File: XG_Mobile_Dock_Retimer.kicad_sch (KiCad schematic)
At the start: 273 parts, among them J1 5-1775443-8, J13 39301240, J14 469911008, J2 20455-040E-76, J3 20455-040E-76, J7 CEE016400140111, SW1 SW_Push, U1 DS160PT801ACBR, U2 TPS7A8400ARGRR, U7 TPS7A8400ARGRR

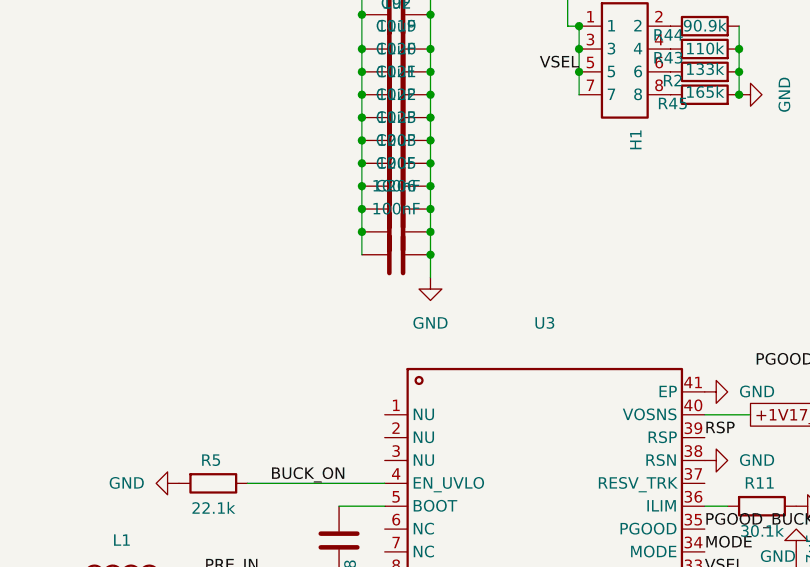
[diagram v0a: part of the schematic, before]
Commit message: ee
eee
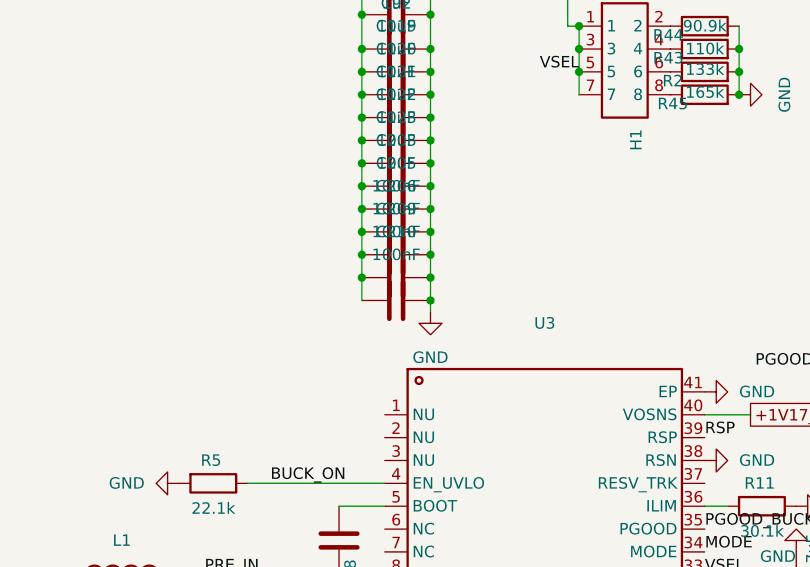
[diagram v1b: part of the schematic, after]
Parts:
- added C209, C210: 100nF, Capacitor_SMD:C_0201_0603Metric, symbol Device:C
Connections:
- net +1V17_2: now also C209.2, C210.2
- net GND: now also C209.1, C210.1

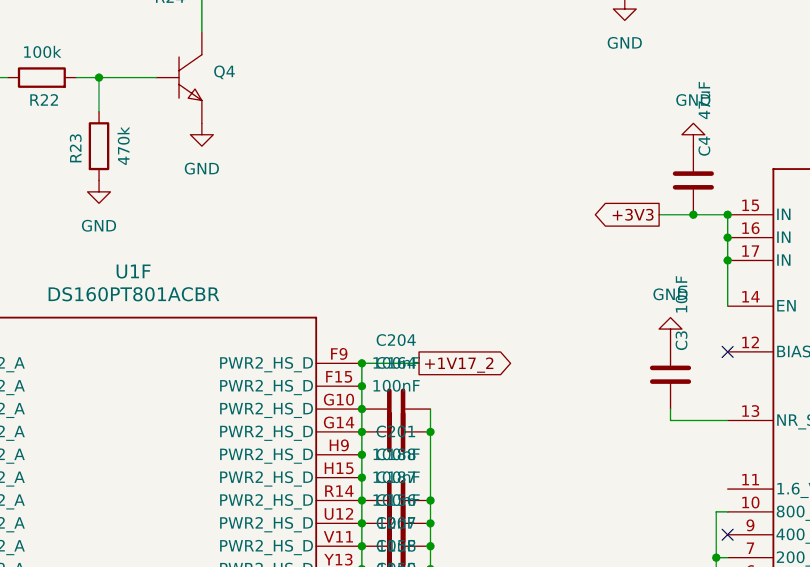
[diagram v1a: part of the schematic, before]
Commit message: eeee
eee
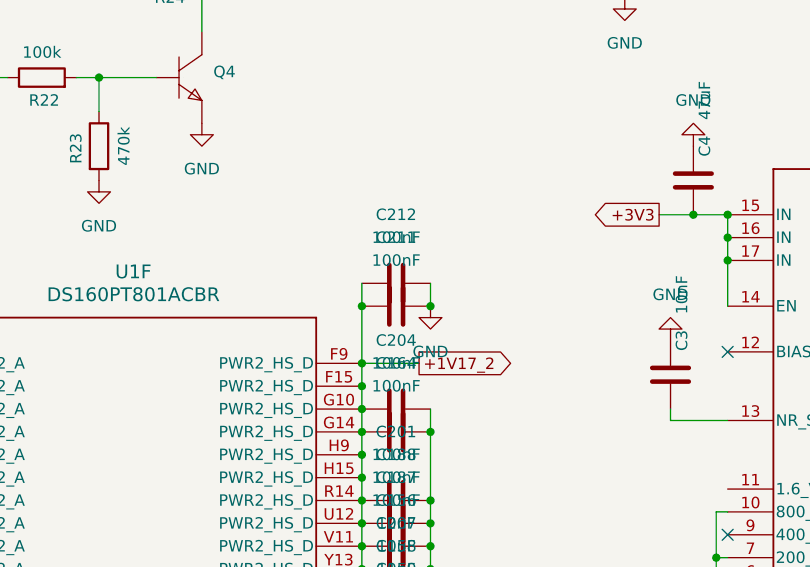
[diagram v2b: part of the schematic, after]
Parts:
- added C211, C212: 100nF, Capacitor_SMD:C_0201_0603Metric, symbol Device:C
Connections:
- net +1V17_2: now also C211.2, C212.2
- net GND: now also C211.1, C212.1

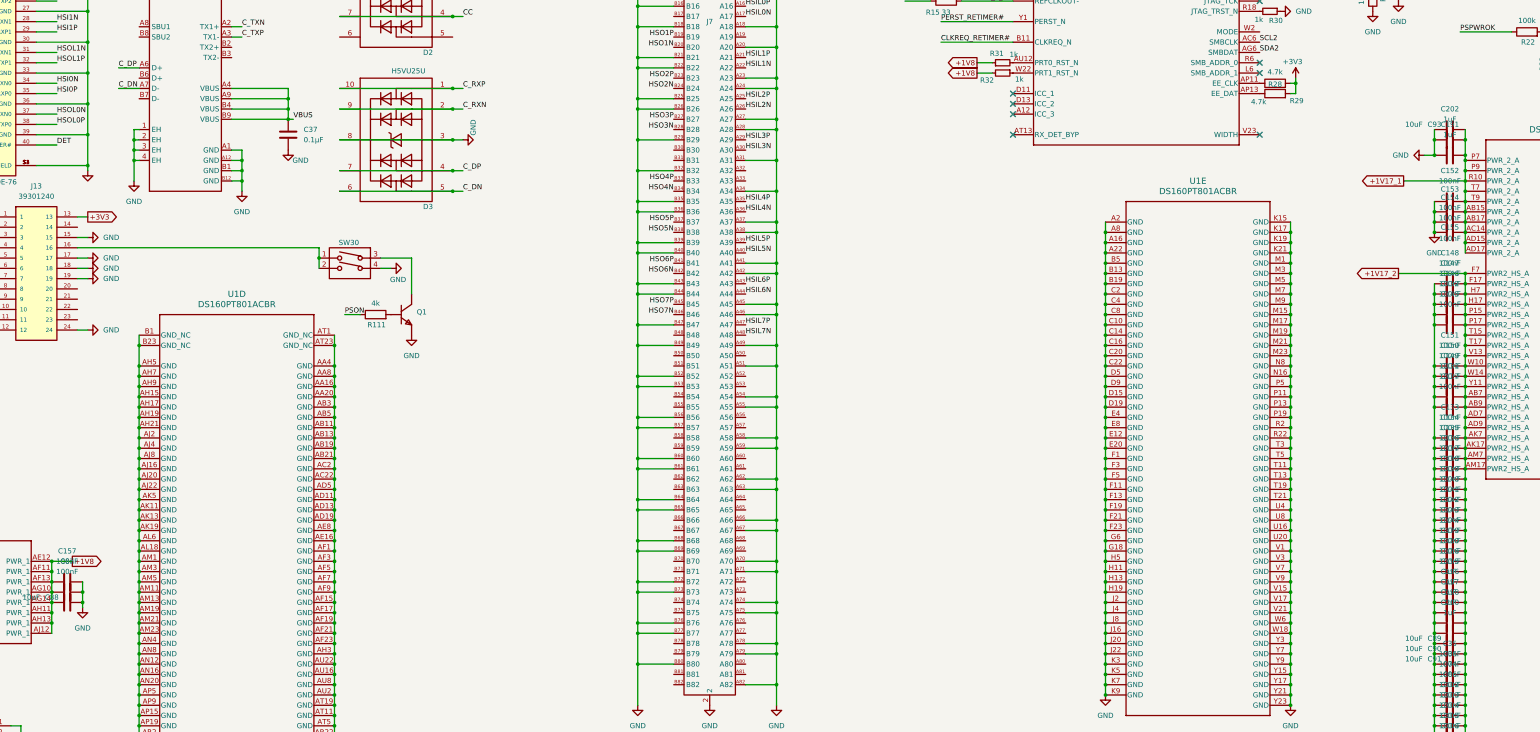
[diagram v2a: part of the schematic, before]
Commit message: eeeeee
eeeeee
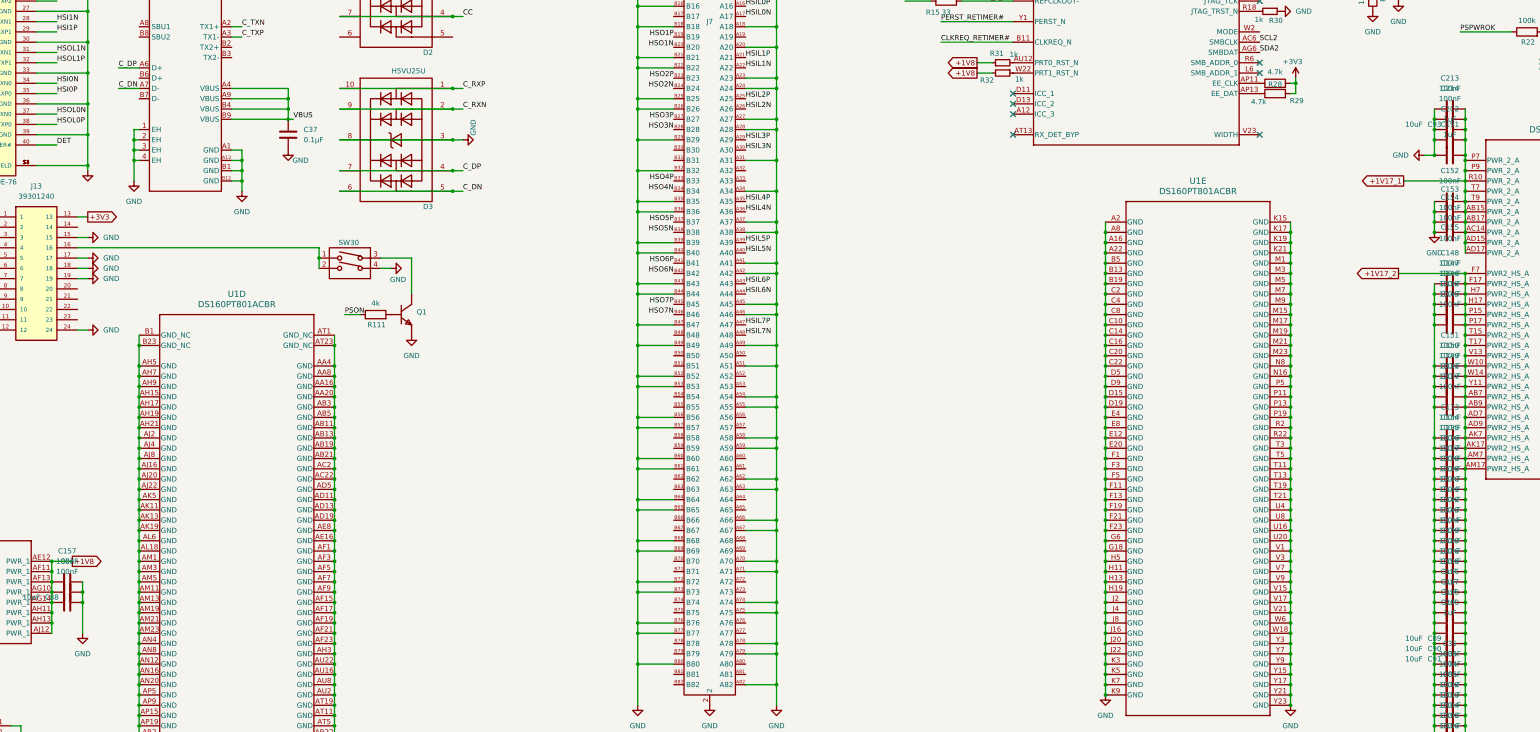
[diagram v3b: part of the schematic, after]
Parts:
- added C213, C214: 100nF, Capacitor_SMD:C_0201_0603Metric, symbol Device:C
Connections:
- net +1V17_1: now also C213.1, C214.1
- net GND: now also C213.2, C214.2

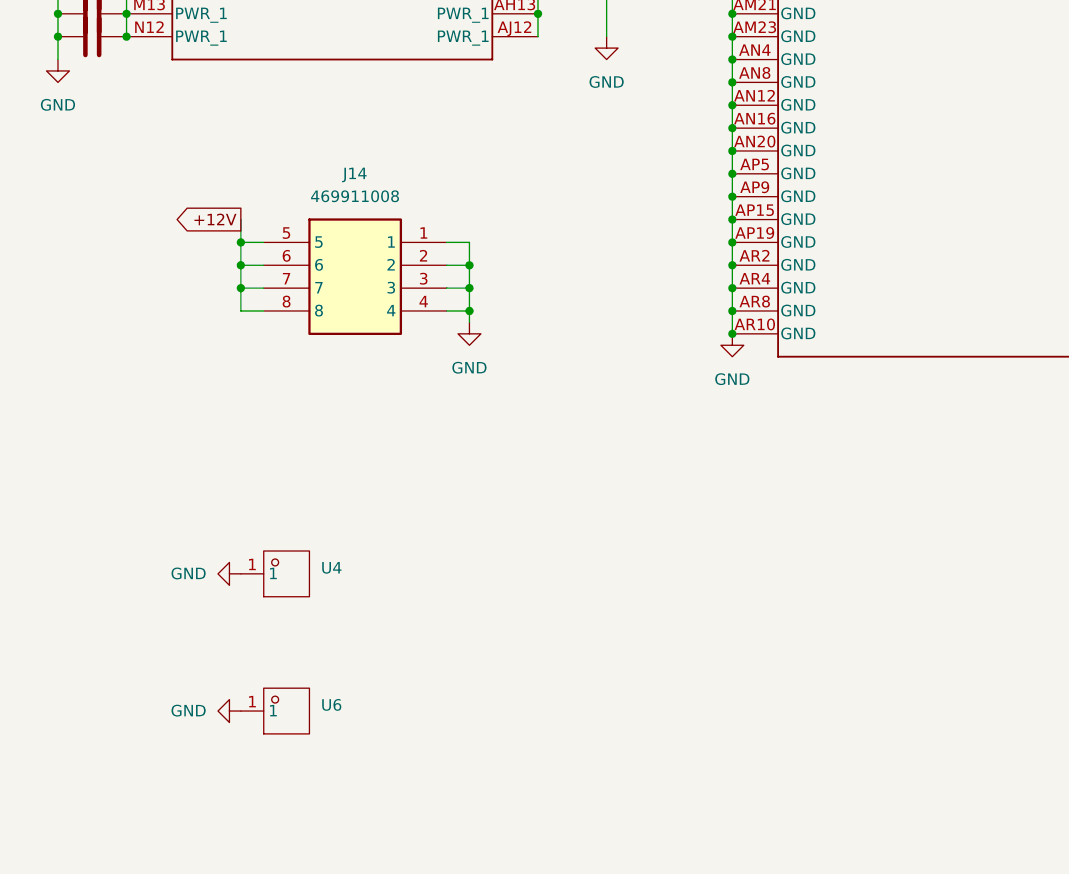
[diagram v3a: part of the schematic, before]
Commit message: eeeee
eeeee
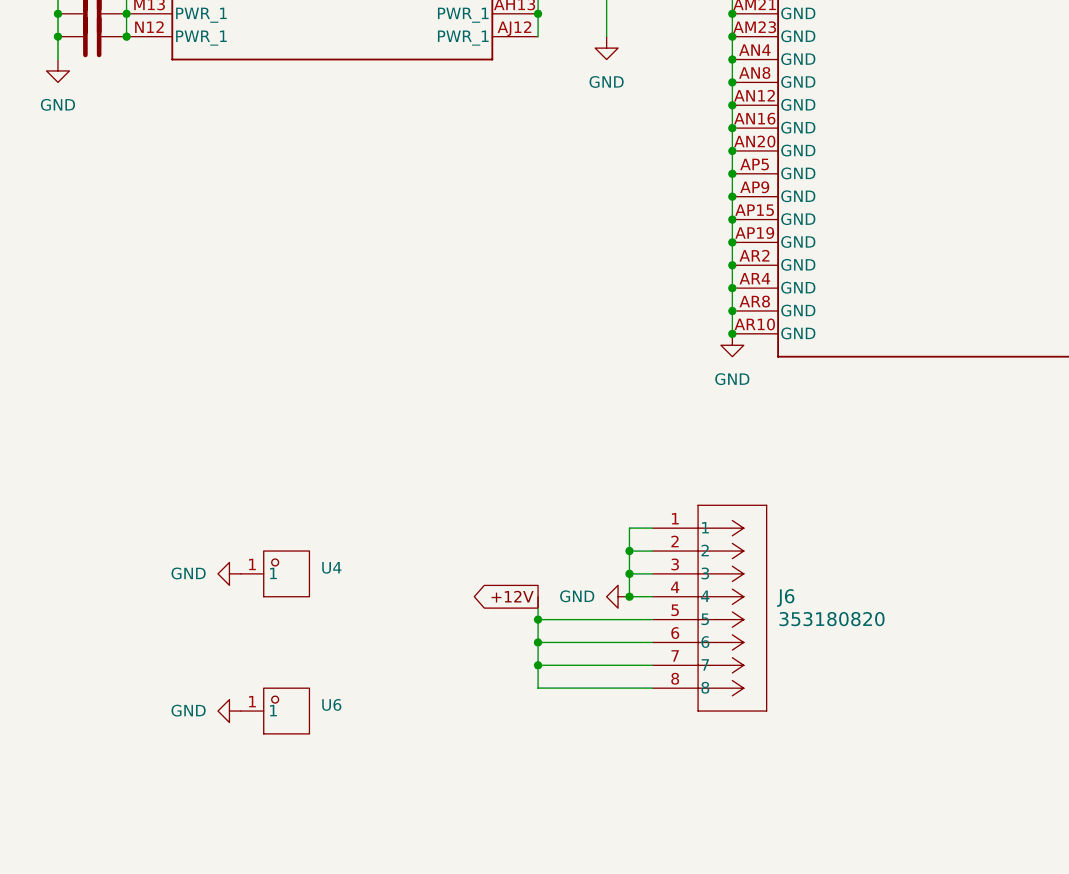
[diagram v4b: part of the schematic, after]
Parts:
- removed J14: 469911008, 469911008:CON_469911008, symbol 3-1775099-2:3-1775099-2
- added J6: 353180820, 353180820:CONN_SD-35318-xxxx_08_MOL, symbol 353180820:353180820
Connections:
- net +12V: now also J6.5, J6.6, J6.7, J6.8
- net GND: now also J6.1, J6.2, J6.3, J6.4

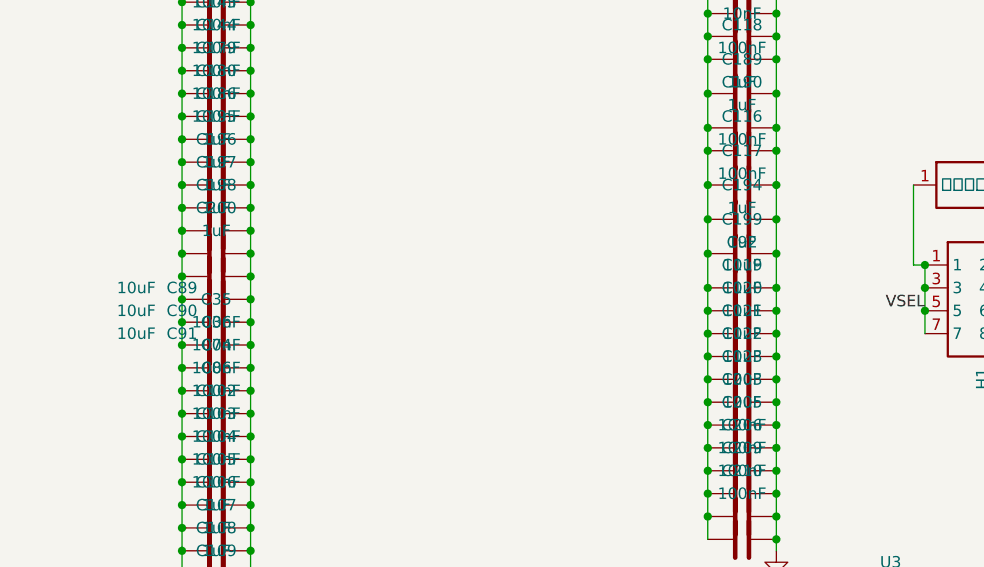
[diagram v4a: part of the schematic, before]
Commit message: eeeee
eeeee
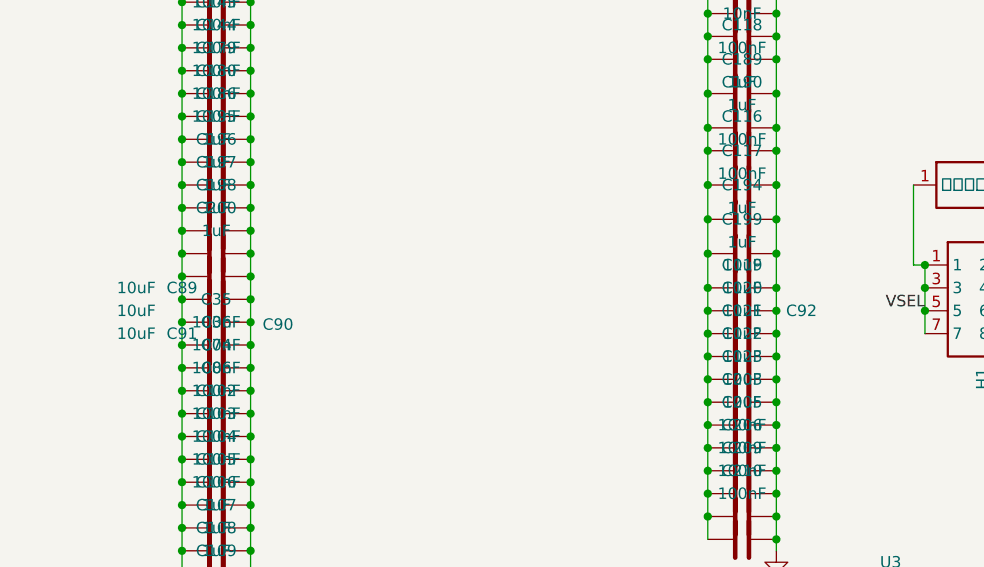
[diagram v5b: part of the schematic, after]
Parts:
- C92: footprint Capacitor_SMD:C_0402_1005Metric -> Capacitor_SMD:C_0805_2012Metric; LCSC C15525 -> C15850; Part_Number CL05A106MQ5NUNC -> CL21A106KAYNNNE
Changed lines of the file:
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@@
 		(on_board yes)
 		(dnp no)
-		(fields_autoplaced yes)
 		(property "Reference" "C35"
 			(at 419.1 241.3 90)
@@
 		(on_board yes)
 		(dnp no)
-		(fields_autoplaced yes)
 		(property "Reference" "C92"
-			(at 477.52 234.95 90)
+			(at 484.124 242.57 90)
 			(effects
 				(font
@@
 			)
 		)
-		(property "Footprint" "Capacitor_SMD:C_0402_1005Metric"
+		(property "Footprint" "Capacitor_SMD:C_0805_2012Metric"
 			(at 473.71 243.5352 0)
 			(effects
@@
 			)
 		)
-		(property "LCSC" "C15525"
+		(property "LCSC" "C15850"
 			(at 477.52 242.57 0)
 			(effects
@@
 			)
 		)
-		(property "Part_Number" "CL05A106MQ5NUNC"
+		(property "Part_Number" "CL21A106KAYNNNE"
 			(at 477.52 242.57 0)
 			(effects
@@
 		(on_board yes)
 		(dnp no)
-		(fields_autoplaced yes)
 		(property "Reference" "C36"
 			(at 419.1 243.84 90)
@@
 		(dnp no)
 		(property "Reference" "C90"
-			(at 415.29 242.57 90)
+			(at 425.958 244.094 90)
 			(effects
 				(font

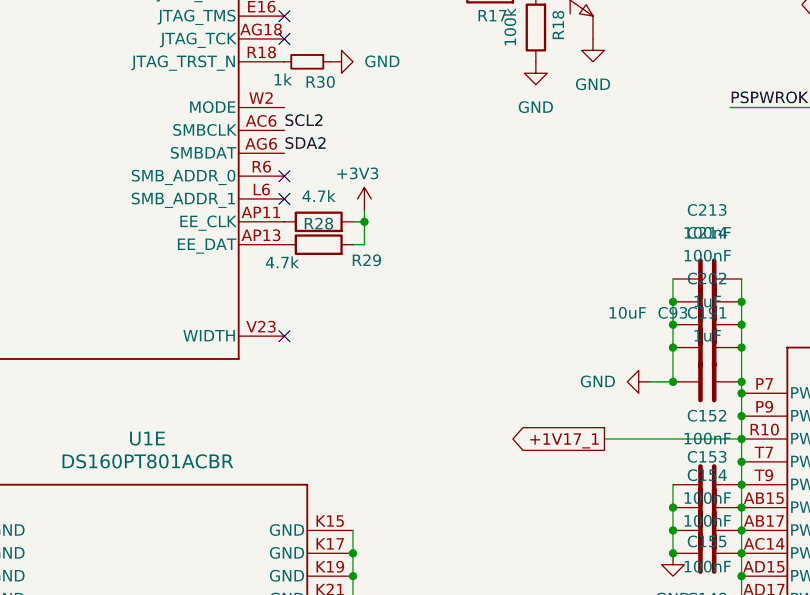
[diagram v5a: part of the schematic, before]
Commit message: eeee
eeee
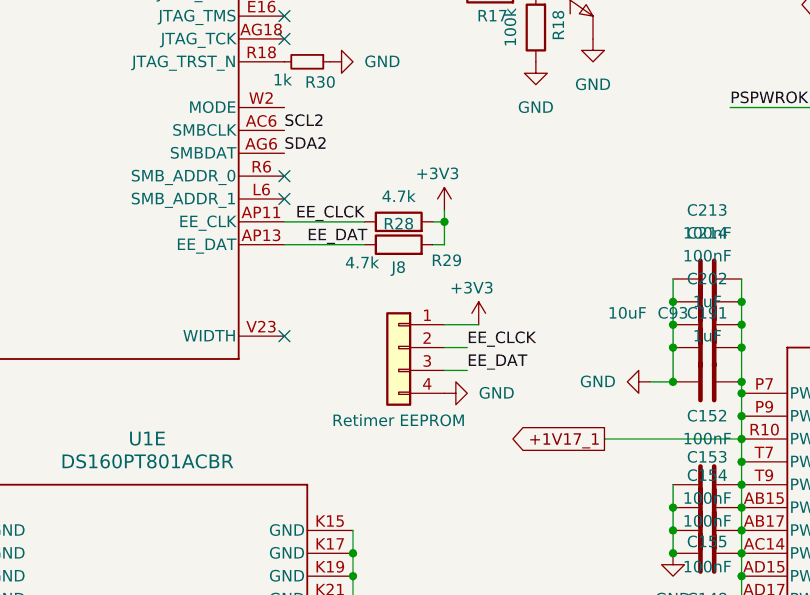
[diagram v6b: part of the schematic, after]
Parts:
- added J8: Retimer EEPROM, Connector_PinHeader_2.54mm:PinHeader_1x04_P2.54mm_Vertical, symbol Connector_Generic:Conn_01x04
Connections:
- net +3V3: now also J8.1 (Pin_1)
- net GND: now also J8.4 (Pin_4)
- net EE_DAT: now reaches R29.1, U1.AP13 (EE_DAT)
- net EE_DAT: now also J8.3 (Pin_3)
- net EE_CLCK: now reaches R28.1, U1.AP11 (EE_CLK)
- net EE_CLCK: now also J8.2 (Pin_2)
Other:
- moved on the sheet: R28, R29

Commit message: eeeeeeee
eeeee
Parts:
- H1, H2: LCSC (none) -> C492421; LCSC Part Name 2x4P 间距:2.54mm 方针 直插 -> (none); Manufacturer Part PZ254V-12-8P -> (none); Part_Number (none) -> PZ254V-12-8P; Supplier LCSC -> (none); Supplier Part C492421 -> (none)
- J4, J5: LCSC (none) -> C5305; LCSC Part Name 2.54mm 开顶式 -> (none); Manufacturer Part 2.54短路帽开口 -> (none); Part_Number (none) -> 2.54短路帽开口; Supplier LCSC -> (none); Supplier Part C5305 -> (none)
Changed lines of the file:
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@@
 			)
 		)
-		(property "Manufacturer Part" "2.54短路帽开口"
+		(property "Part_Number" "2.54短路帽开口"
 			(at 542.29 226.06 0)
 			(effects
@@
 			)
 		)
-		(property "Supplier Part" "C5305"
-			(at 542.29 226.06 0)
-			(effects
-				(font
-					(size 1.27 1.27)
-				)
-				(hide yes)
-			)
-		)
-		(property "Supplier" "LCSC"
-			(at 542.29 226.06 0)
-			(effects
-				(font
-					(size 1.27 1.27)
-				)
-				(hide yes)
-			)
-		)
-		(property "LCSC Part Name" "2.54mm 开顶式"
+		(property "LCSC" "C5305"
 			(at 542.29 226.06 0)
 			(effects
@@
 			)
 		)
-		(property "Manufacturer Part" "PZ254V-12-8P"
+		(property "Part_Number" "PZ254V-12-8P"
 			(at 502.92 241.3 0)
 			(effects
@@
 			)
 		)
-		(property "Supplier Part" "C492421"
-			(at 502.92 241.3 0)
-			(effects
-				(font
-					(size 1.27 1.27)
-				)
-				(hide yes)
-			)
-		)
-		(property "Supplier" "LCSC"
-			(at 502.92 241.3 0)
-			(effects
-				(font
-					(size 1.27 1.27)
-				)
-				(hide yes)
-			)
-		)
-		(property "LCSC Part Name" "2x4P 间距:2.54mm 方针 直插"
+		(property "LCSC" "C492421"
 			(at 502.92 241.3 0)
 			(effects
@@
 			)
 		)
-		(property "Manufacturer Part" "2.54短路帽开口"
+		(property "Part_Number" "2.54短路帽开口"
 			(at 504.19 228.6 0)
 			(effects
@@
 			)
 		)
-		(property "Supplier Part" "C5305"
-			(at 504.19 228.6 0)
-			(effects
-				(font
-					(size 1.27 1.27)
-				)
-				(hide yes)
-			)
-		)
-		(property "Supplier" "LCSC"
-			(at 504.19 228.6 0)
-			(effects
-				(font
-					(size 1.27 1.27)
-				)
-				(hide yes)
-			)
-		)
-		(property "LCSC Part Name" "2.54mm 开顶式"
+		(property "LCSC" "C5305"
 			(at 504.19 228.6 0)
 			(effects
@@
 			)
 		)
-		(property "Manufacturer Part" "PZ254V-12-8P"
+		(property "Part_Number" "PZ254V-12-8P"
 			(at 537.21 242.57 0)
 			(effects
@@
 			)
 		)
-		(property "Supplier Part" "C492421"
-			(at 537.21 242.57 0)
-			(effects
-				(font
-					(size 1.27 1.27)
-				)
-				(hide yes)
-			)
-		)
-		(property "Supplier" "LCSC"
-			(at 537.21 242.57 0)
-			(effects
-				(font
-					(size 1.27 1.27)
-				)
-				(hide yes)
-			)
-		)
-		(property "LCSC Part Name" "2x4P 间距:2.54mm 方针 直插"
+		(property "LCSC" "C492421"
 			(at 537.21 242.57 0)
 			(effects
